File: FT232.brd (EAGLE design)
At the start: 100 x 80 mm, 17 parts, among them J1 USB, J2 CON, U1 FT232, Y1 CRYSTAL

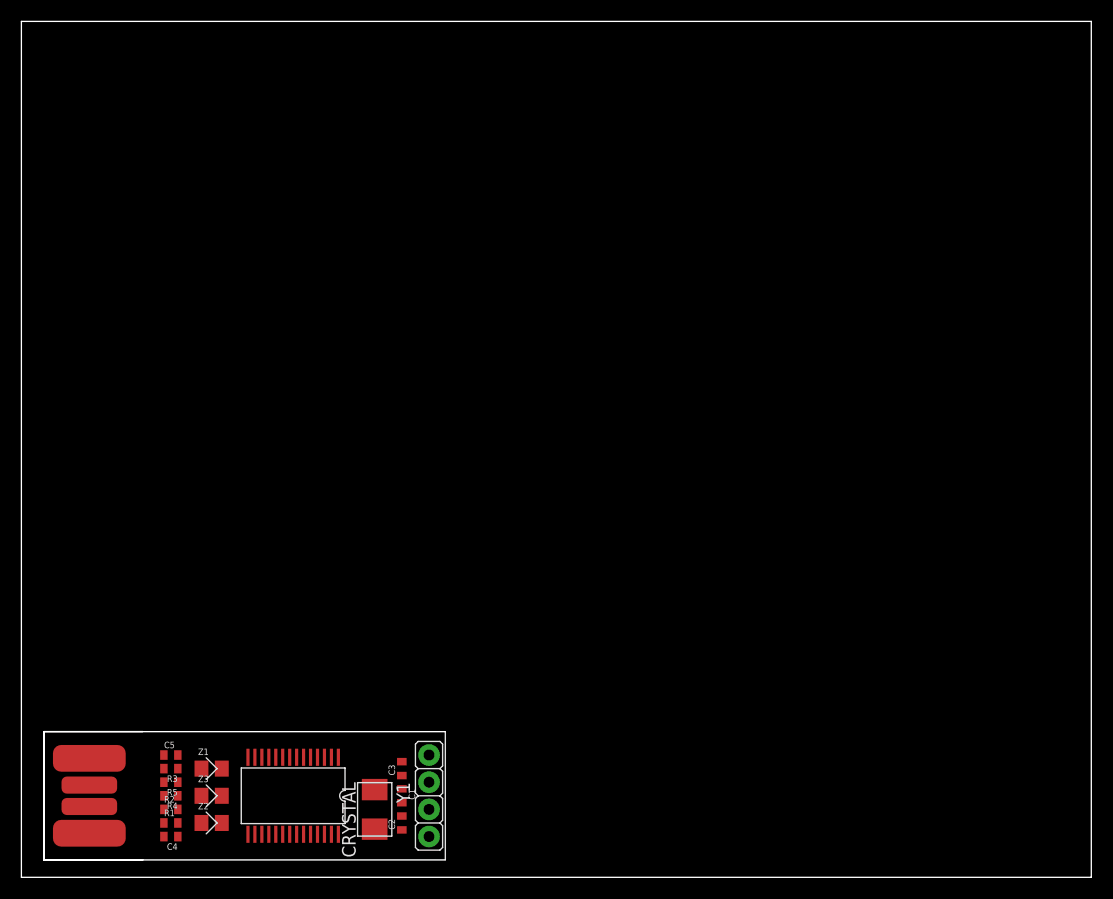
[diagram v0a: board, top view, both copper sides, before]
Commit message: 第二次布线尝试
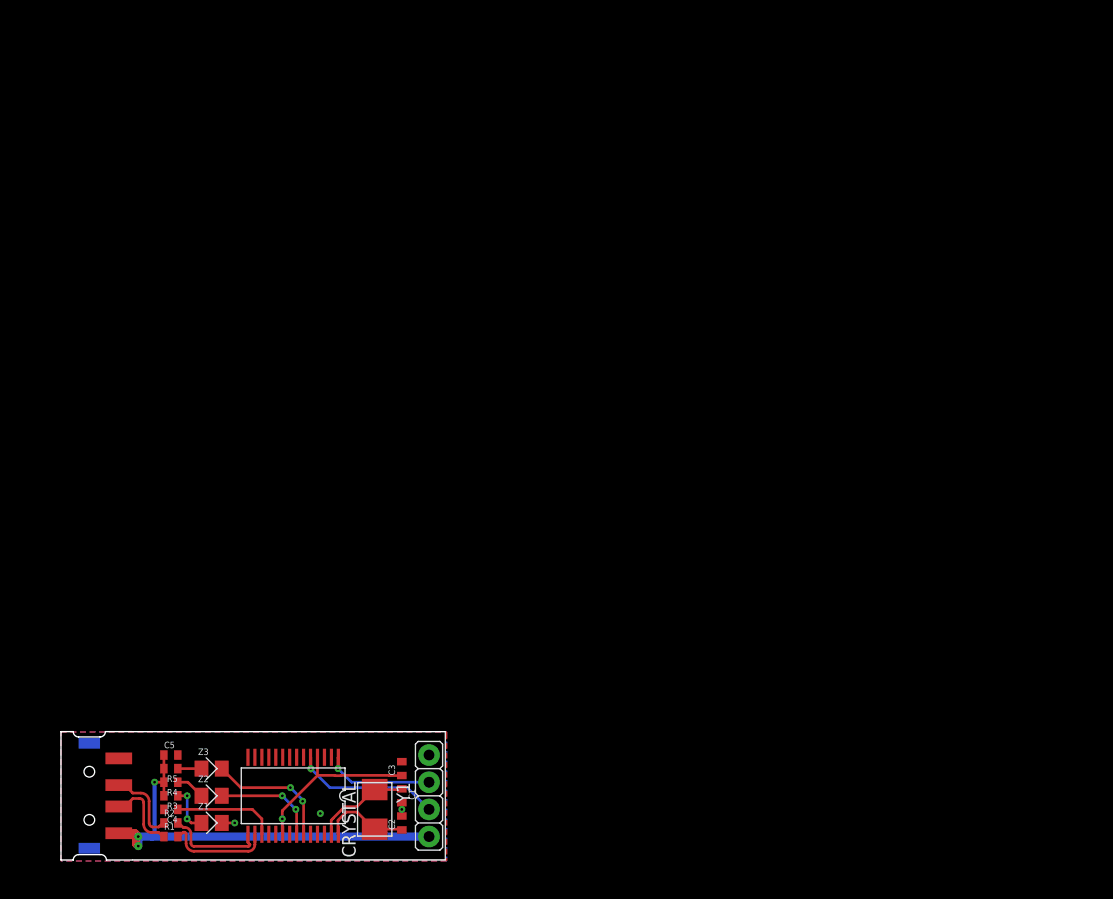
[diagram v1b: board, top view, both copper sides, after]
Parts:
- J1: value USB -> USBA; device FT232:USB_SMD -> FT232:USB_A
- moved Z1 5.08 mm to (17.8, 5.08)
- moved R3 2.54 mm to (14.0, 7.62)
- moved Z2 2.54 mm to (17.8, 7.62)
- moved Z3 2.54 mm to (17.8, 10.2)
- moved C4 2.54 mm to (14.0, 6.35)
- moved R4 1.27 mm to (14.0, 8.89)
- moved R1 1.27 mm to (14.0, 3.81)
- moved R2 1.27 mm to (14.0, 5.08)
- moved R5 1.27 mm to (14.0, 10.2)
- turned J1 to 270 degrees
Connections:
- net N$1 renamed D_N
- net N$2 renamed D_P
- net +5V: now also J1.VBUS; no longer J1.VCC
- net GND: now also J1.GND1, J1.GND2
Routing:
- net +5V: track 0.00 -> 59.6 mm, vias 0 -> 4
- net RXD: track 0.00 -> 14.0 mm, vias 0 -> 1
- net N$8: track 0.00 -> 12.0 mm, vias 0 -> 2
- net TXD: track 0.00 -> 10.2 mm, vias 0 -> 1
- net D_N: track 0.00 -> 9.85 mm
- net N$9: track 0.00 -> 9.81 mm, vias 0 -> 2
- net N$7: track 0.00 -> 9.67 mm
- net D_P: track 0.00 -> 9.28 mm
- net N$6: track 0.00 -> 9.15 mm
- net N$5: track 0.00 -> 8.30 mm
- net N$4: track 0.00 -> 7.19 mm
- net N$3: track 0.00 -> 7.19 mm
- net N$12: track 0.00 -> 4.53 mm, vias 0 -> 2
- net N$11: track 0.00 -> 2.74 mm
- net GND: track 0.00 -> 2.45 mm, vias 0 -> 3
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- added copper zone on layer 1, net GND
- added copper zone on layer 16, net GND
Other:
- board size 100 x 80 mm -> 29.2 x 12 mm
